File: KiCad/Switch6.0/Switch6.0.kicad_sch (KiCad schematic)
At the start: 45 parts, among them Q1 BD139, Q2 IXTH90P10P, Q4 BD139, Q5A1 BSC340N08NS3G, Q6 BD139

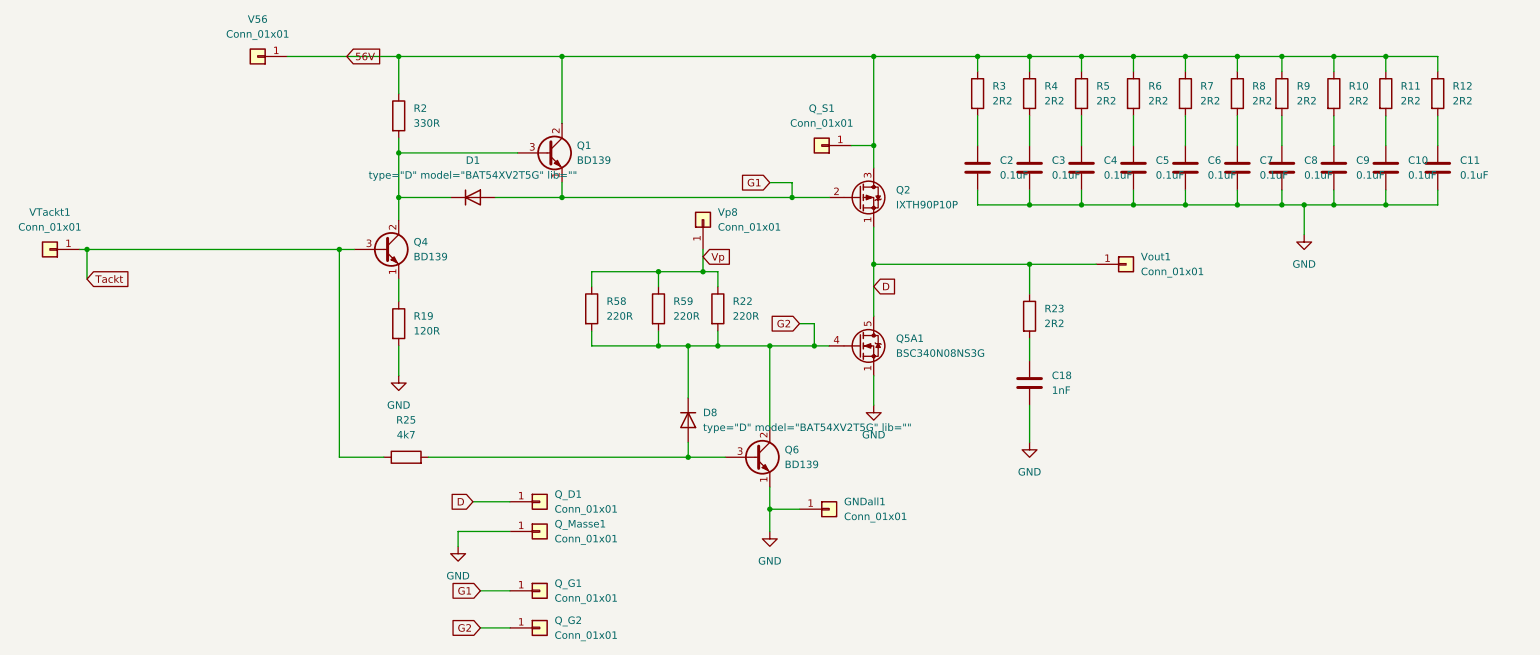
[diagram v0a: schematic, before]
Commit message: Switch Platine
Platine 0.2 Entwurf mit OpV
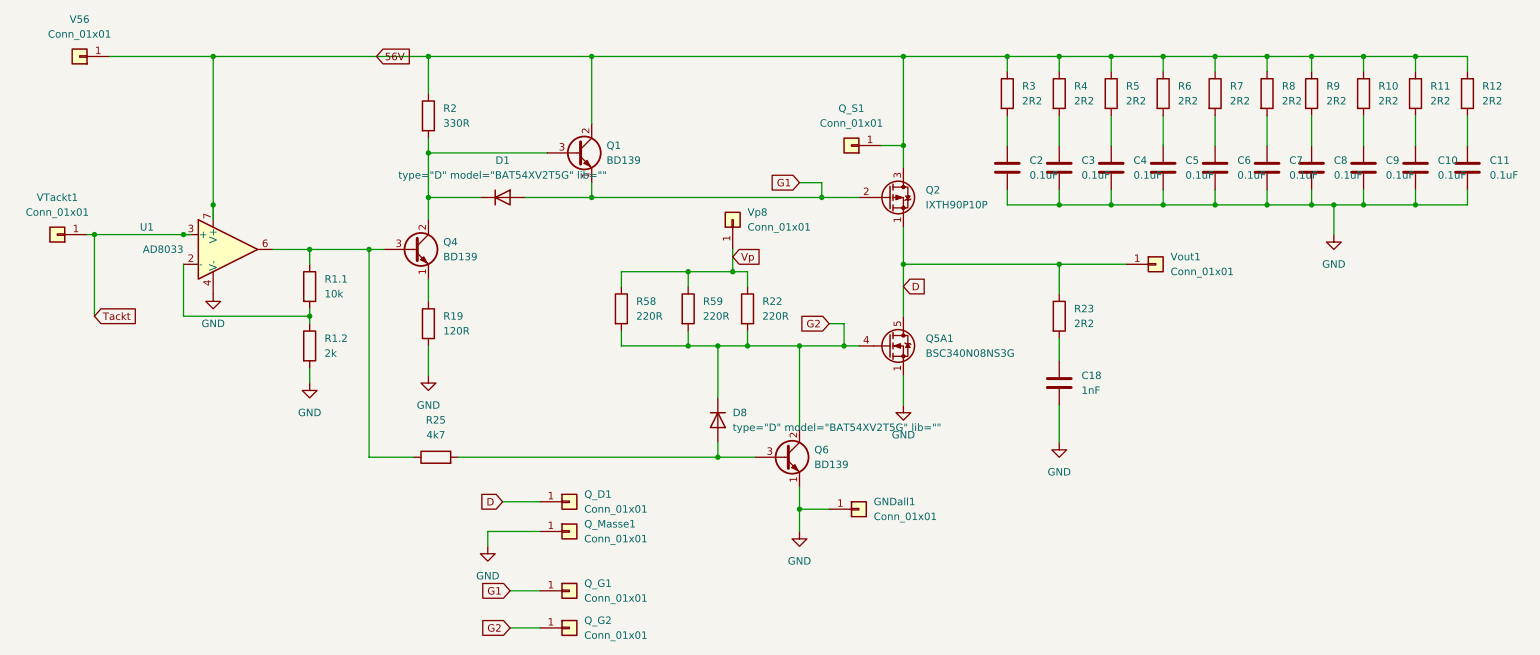
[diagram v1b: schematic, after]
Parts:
- added R1.1: 10k, Resistor_SMD:R_0805_2012Metric, symbol Device:R
- added R1.2: 2k, Resistor_SMD:R_0805_2012Metric, symbol Device:R
- added U1: AD8033, Package_SO:SOIC-8_3.9x4.9mm_P1.27mm, symbol Amplifier_Operational:AD8001AR
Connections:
- net 56V: now also U1.7 (V+)
- net GND: now also R1.2.2, U1.4 (V-)
- net Tackt: now also U1.3 (+); no longer Q4.3 (B), R25.1
- new net: Q4.3 (B), R1.1.1, R25.1, U1.6
- new net: R1.1.2, R1.2.1, U1.2 (-)
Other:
- moved on the sheet: C10, C11, C18, C2, C3, C4, C5, C6, C7, C8, C9, D1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
